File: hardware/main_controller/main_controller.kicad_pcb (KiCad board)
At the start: 2 copper layers, 25 x 25 mm, 12 parts, among them J1 Conn_01x04, U1 QRE1113

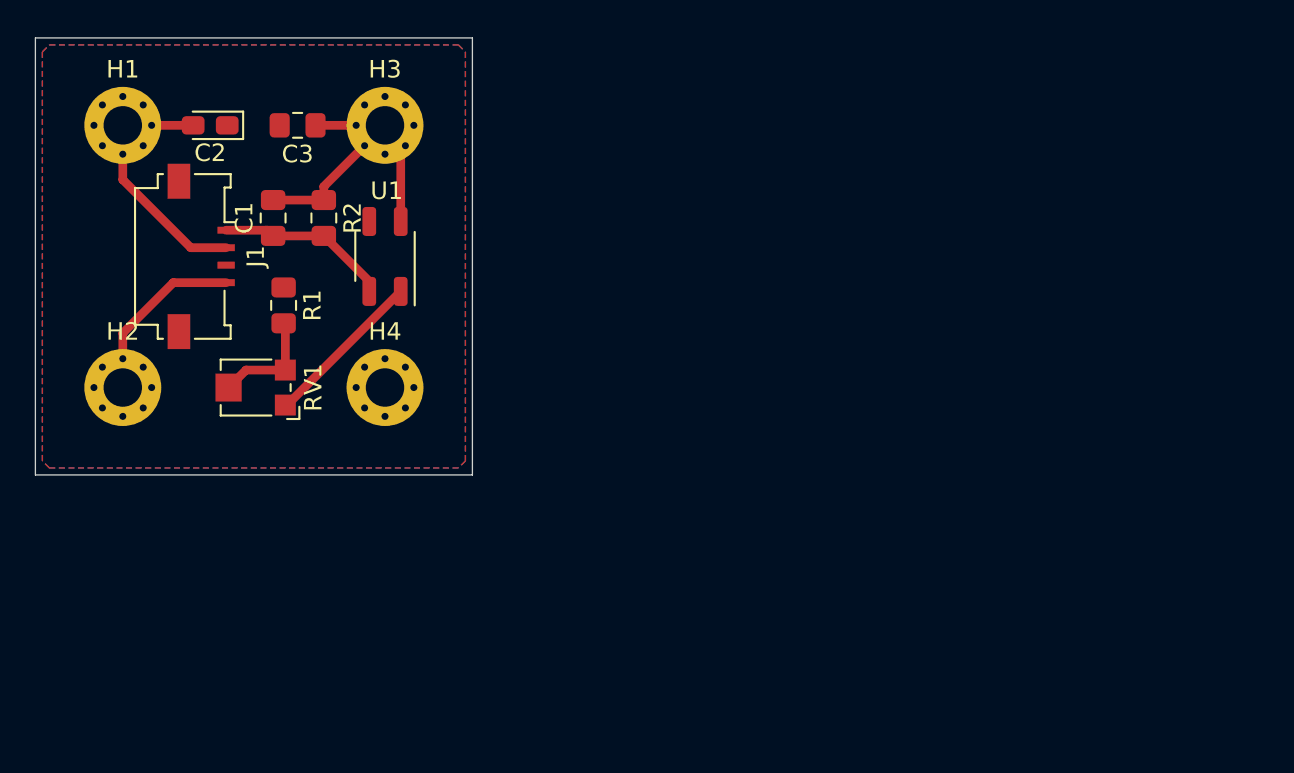
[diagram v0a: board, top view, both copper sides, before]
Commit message: Created main controller. Prototypes finished.
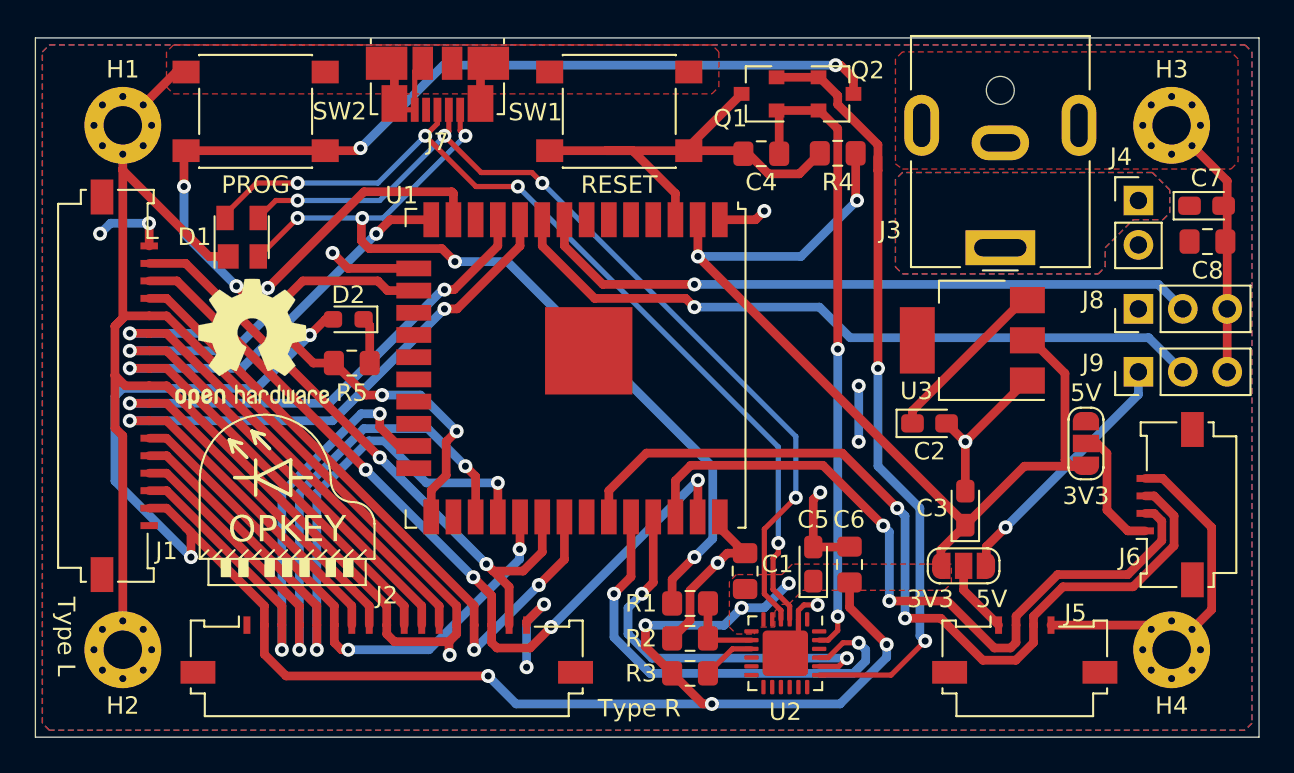
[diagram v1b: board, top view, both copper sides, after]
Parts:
- removed RV1: 200, Potentiometer_SMD:Potentiometer_Bourns_TC33X_Vertical
- added C4: 100nF, Capacitor_SMD:C_0805_2012Metric_Pad1.15x1.40mm_HandSolder, F.Cu at (71.5, 36.6)
- added C5: 10uF, Capacitor_Tantalum_SMD:CP_EIA-2012-15_AVX-P_Pad1.30x1.05mm_HandSolder, F.Cu at (74.5, 60.1)
- added C6: 100nF, Capacitor_SMD:C_0805_2012Metric_Pad1.15x1.40mm_HandSolder, F.Cu at (76.6, 60.1)
- added C7: 10uF, Capacitor_Tantalum_SMD:CP_EIA-2012-15_AVX-P_Pad1.30x1.05mm_HandSolder, F.Cu at (97.0, 39.6)
- added C8: 100nF, Capacitor_SMD:C_0805_2012Metric_Pad1.15x1.40mm_HandSolder, F.Cu at (97.0, 41.6)
- added D1: SP0503BAHT, Package_TO_SOT_SMD:SOT-143, F.Cu at (41.8, 41.4)
- added D2: LED_Blue_2V6_2mA, LED_SMD:LED_0603_1608Metric_Pad1.05x0.95mm_HandSolder, F.Cu at (47.9, 46.1)
- added J2: Conn_01x17, Connector_FFC-FPC:Molex_200528-0170_1x17-1MP_P1.00mm_Horizontal, F.Cu at (50.1, 64.5)
- added J3: Barrel_Jack, Connector_BarrelJack:BarrelJack_CUI_PJ-063AH_Horizontal, F.Cu at (85.2, 42.0)
- added J4: Conn_01x02, Connector_PinHeader_2.54mm:PinHeader_1x02_P2.54mm_Vertical, F.Cu at (93.1, 39.3)
- added J5: Conn_01x04, Connector_FFC-FPC:Molex_200528-0040_1x04-1MP_P1.00mm_Horizontal, F.Cu at (86.6, 64.5)
- added J6: Conn_01x04, Connector_FFC-FPC:Molex_200528-0040_1x04-1MP_P1.00mm_Horizontal, F.Cu at (94.4, 56.7)
- added J7: USB_B_Micro, Connector_USB:USB_Micro-B_Molex_47346-0001, F.Cu at (53.0, 32.6)
- added J8: Conn_01x03, Connector_PinHeader_2.54mm:PinHeader_1x03_P2.54mm_Vertical, F.Cu at (93.1, 45.5)
- added J9: Conn_01x03, Connector_PinHeader_2.54mm:PinHeader_1x03_P2.54mm_Vertical, F.Cu at (93.1, 49.1)
- added JP1: SolderJumper_3_Open, Jumper:SolderJumper-3_P1.3mm_Open_RoundedPad1.0x1.5mm_NumberLabels, F.Cu at (83.1, 60.2)
- added JP2: SolderJumper_3_Open, Jumper:SolderJumper-3_P1.3mm_Open_RoundedPad1.0x1.5mm_NumberLabels, F.Cu at (90.1, 53.2)
- added Q1: 2N7002, Package_TO_SOT_SMD:SOT-23, F.Cu at (71.4, 33.2)
- added Q2: 2N7002, Package_TO_SOT_SMD:SOT-23, F.Cu at (75.8, 33.2)
- added R3: 4k7, Resistor_SMD:R_0805_2012Metric_Pad1.15x1.40mm_HandSolder, F.Cu at (67.5, 66.3)
- added R4: 10k, Resistor_SMD:R_0805_2012Metric_Pad1.15x1.40mm_HandSolder, F.Cu at (75.9, 36.6)
- added R5: 1k, Resistor_SMD:R_0805_2012Metric_Pad1.15x1.40mm_HandSolder, F.Cu at (48.1, 48.6)
- added REF**: OSHW-Logo2_9.8x8mm_SilkScreen, Symbol:OSHW-Logo2_9.8x8mm_SilkScreen, F.Cu at (42.4, 47.5)
- added REF**: OpKey_Logo, OpKey:OpKey_Logo, F.Cu at (44.4, 56.3)
- added SW1: SW_Push, Button_Switch_SMD:SW_SPST_PTS645, F.Cu at (63.4, 34.2)
- added SW2: SW_Push, Button_Switch_SMD:SW_SPST_PTS645, F.Cu at (42.6, 34.2)
- added U2: CP2104, Package_DFN_QFN:QFN-24-1EP_4x4mm_P0.5mm_EP2.6x2.6mm, F.Cu at (72.9, 65.2)
- added U3: LM1117-3.3, Package_TO_SOT_SMD:SOT-223, F.Cu at (83.6, 47.3)
- C2: value 10uF -> 47µF
- C3: value 100nF -> 47µF; footprint Capacitor_SMD:C_0805_2012Metric_Pad1.15x1.40mm_HandSolder -> Capacitor_Tantalum_SMD:CP_EIA-2012-15_AVX-P_Pad1.30x1.05mm_HandSolder
- J1: value Conn_01x04 -> Conn_01x17; footprint Connector_FFC-FPC:Molex_200528-0040_1x04-1MP_P1.00mm_Horizontal -> Connector_FFC-FPC:Molex_200528-0170_1x17-1MP_P1.00mm_Horizontal
- R1: value 150 -> 24k
- R2: value 10k -> 47k
- U1: value QRE1113 -> ESP32-WROOM-32U; footprint OptoDevice:OnSemi_CASE100CY -> RF_Module:ESP32-WROOM-32U
- moved H4 47.4 mm to (95.0, 65.0)
- moved H3 45.0 mm to (95.0, 35.0)
- moved C2 44.5 mm to (81.2, 52.0), turned to 0 degrees
- moved C3 44.0 mm to (83.2, 56.9), turned to 90 degrees
- moved C1 33.7 mm to (70.6, 60.5)
- moved R2 31.9 mm to (67.5, 64.3), turned to 0 degrees
- moved R1 28.8 mm to (67.5, 62.4), turned to 0 degrees
- moved H2 15.0 mm to (35.0, 65.0)
- moved U1 12.6 mm to (60.9, 48.9), turned to 270 degrees
- moved J1 8.61 mm to (35.6, 49.9)
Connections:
- C1 pad 1: /SENSOR_AUX -> +3V3
- C3 pad 1: GND -> +3V3
- C3 pad 2: +5V -> GND
- J1 pad 1: /SENSOR_AUX -> +5V
- J1 pad 2: GND -> SCLK1
- J1 pad 3: +5V -> SDI1
- J1 pad 4: GND -> SDO1
- R1 pad 1: +5V -> USB_VBUS
- R2 pad 2: /SENSOR_AUX -> Net-(R1-Pad2)
- U1 pad 1: Net-(RV1-Pad1) -> GND
- U1 pad 2: GND -> +3V3
- U1 pad 3: +5V -> EN
- U1 pad 4: /SENSOR_AUX -> Net-(U1-Pad4)
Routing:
- net +3V3: track 0.00 -> 154.8 mm, vias 0 -> 10
- net GND: track 43.3 -> 180.7 mm, vias 0 -> 7
- net GPIO0: track 0.00 -> 72.0 mm, vias 0 -> 6
- net USB_D+: track 0.00 -> 53.2 mm, vias 0 -> 4
- net USB_D-: track 0.00 -> 53.0 mm, vias 0 -> 4
- net USB_VBUS: track 0.00 -> 51.9 mm, vias 0 -> 5
- net I2C_SDA: track 0.00 -> 50.5 mm, vias 0 -> 2
- net HSPI_SCLK: track 0.00 -> 48.7 mm, vias 0 -> 2
- net SDI1: track 0.00 -> 47.7 mm, vias 0 -> 4
- net CS4: track 0.00 -> 46.2 mm, vias 0 -> 2
- net CS5: track 0.00 -> 45.9 mm, vias 0 -> 2
- net RTS: track 0.00 -> 44.9 mm, vias 0 -> 2
- net HSPI_MISO: track 0.00 -> 43.2 mm, vias 0 -> 2
- net I2C_SCL: track 0.00 -> 42.6 mm, vias 0 -> 2
- net HSPI_MOSI: track 0.00 -> 42.0 mm, vias 0 -> 2
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- added copper zone on F.Cu, net +3V3
- added copper zone on F.Cu, net GND
- added copper zone on B.Cu, net Net-(J3-Pad1)
- added copper zone on F.Cu, net Net-(J3-Pad1)
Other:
- board size 25 x 25 mm -> 70 x 40 mm
- board text added: "PROG"
- board text added: "RESET"
- board text added: "Type L"
- board text added: "Type R"
